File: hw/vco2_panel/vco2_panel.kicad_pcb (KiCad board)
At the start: 2 copper layers, 60.6 x 128.5 mm, 24 parts

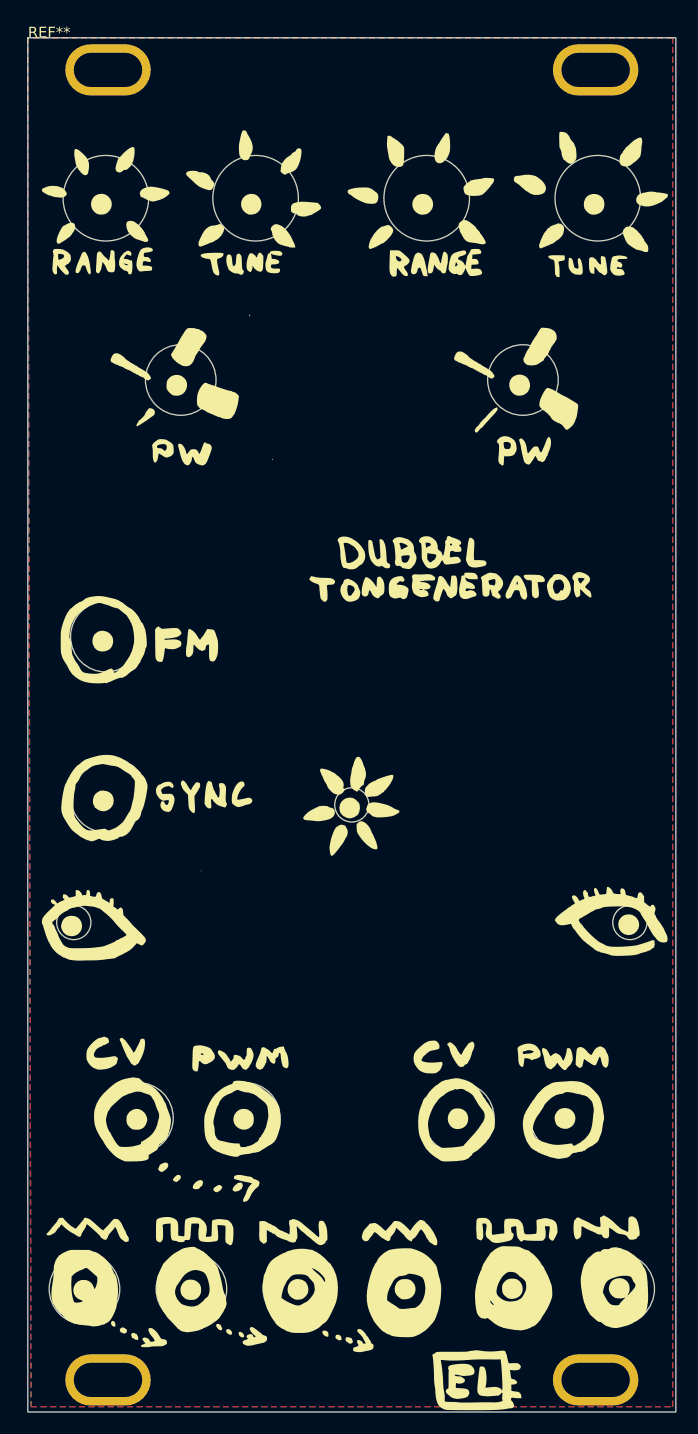
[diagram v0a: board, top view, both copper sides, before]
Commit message: Update VCO2 panel
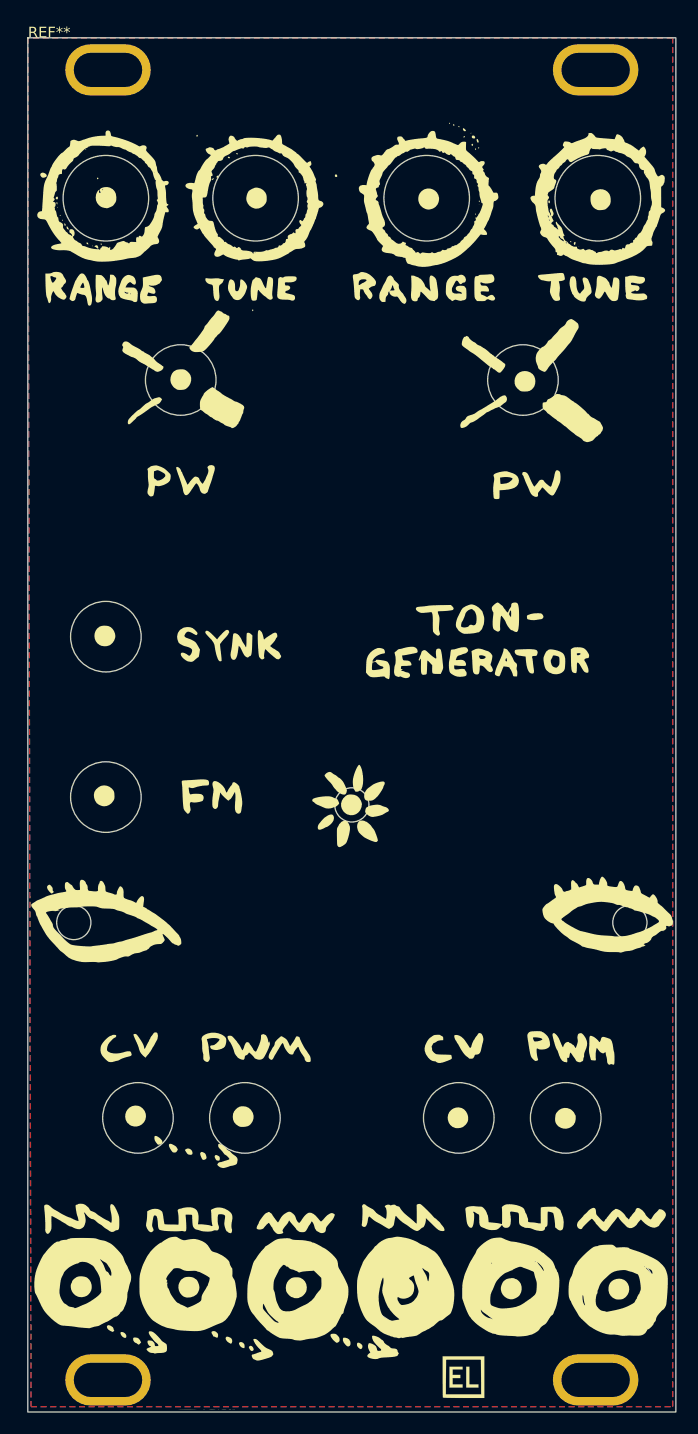
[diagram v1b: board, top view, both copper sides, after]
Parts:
- added G***: LOGO, elemental:elemental-4mm, F.Cu at (120.4, 156.2)
- moved G*** 0.54 mm to (110.2, 95.2)
